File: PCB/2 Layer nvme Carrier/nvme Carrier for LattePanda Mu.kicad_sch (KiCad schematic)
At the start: 8 parts

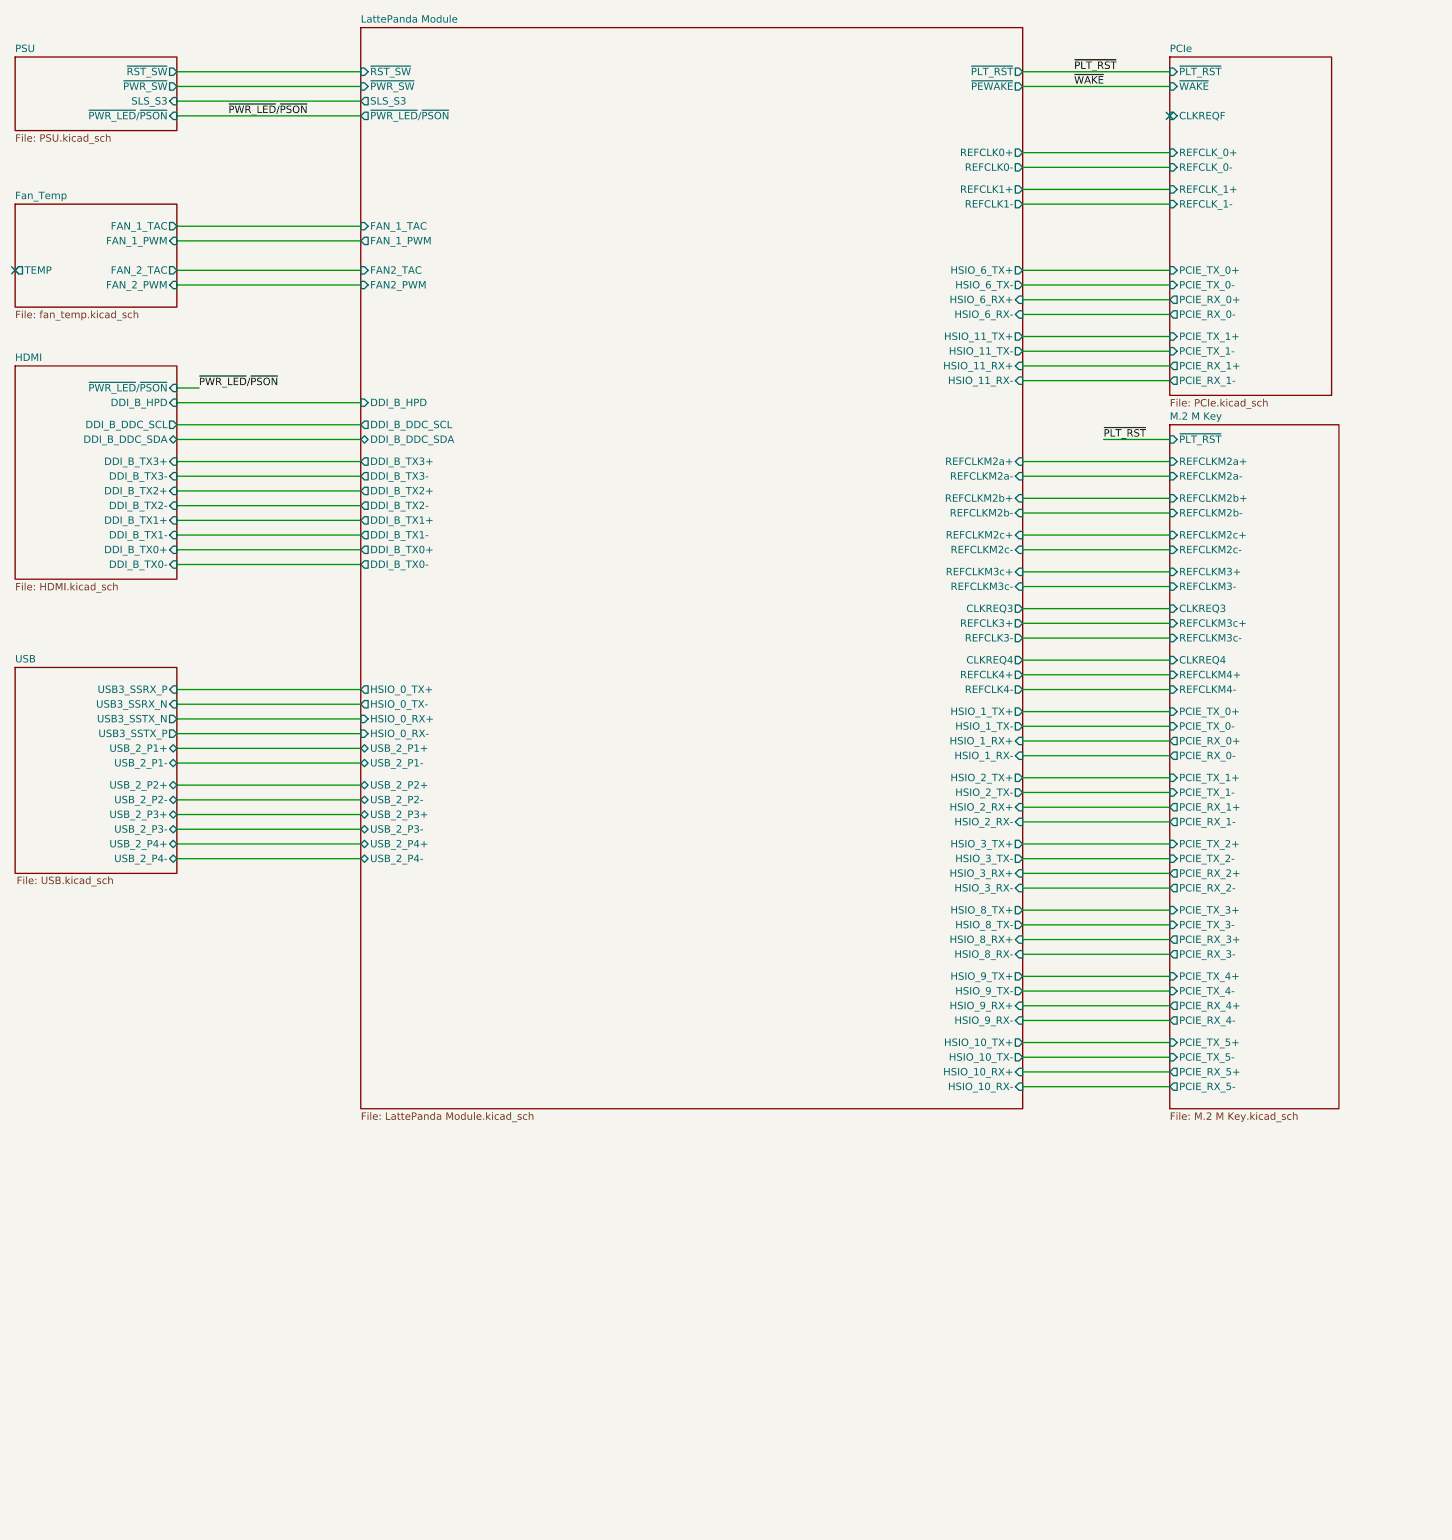
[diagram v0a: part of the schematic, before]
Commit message: Rework started with PCIe
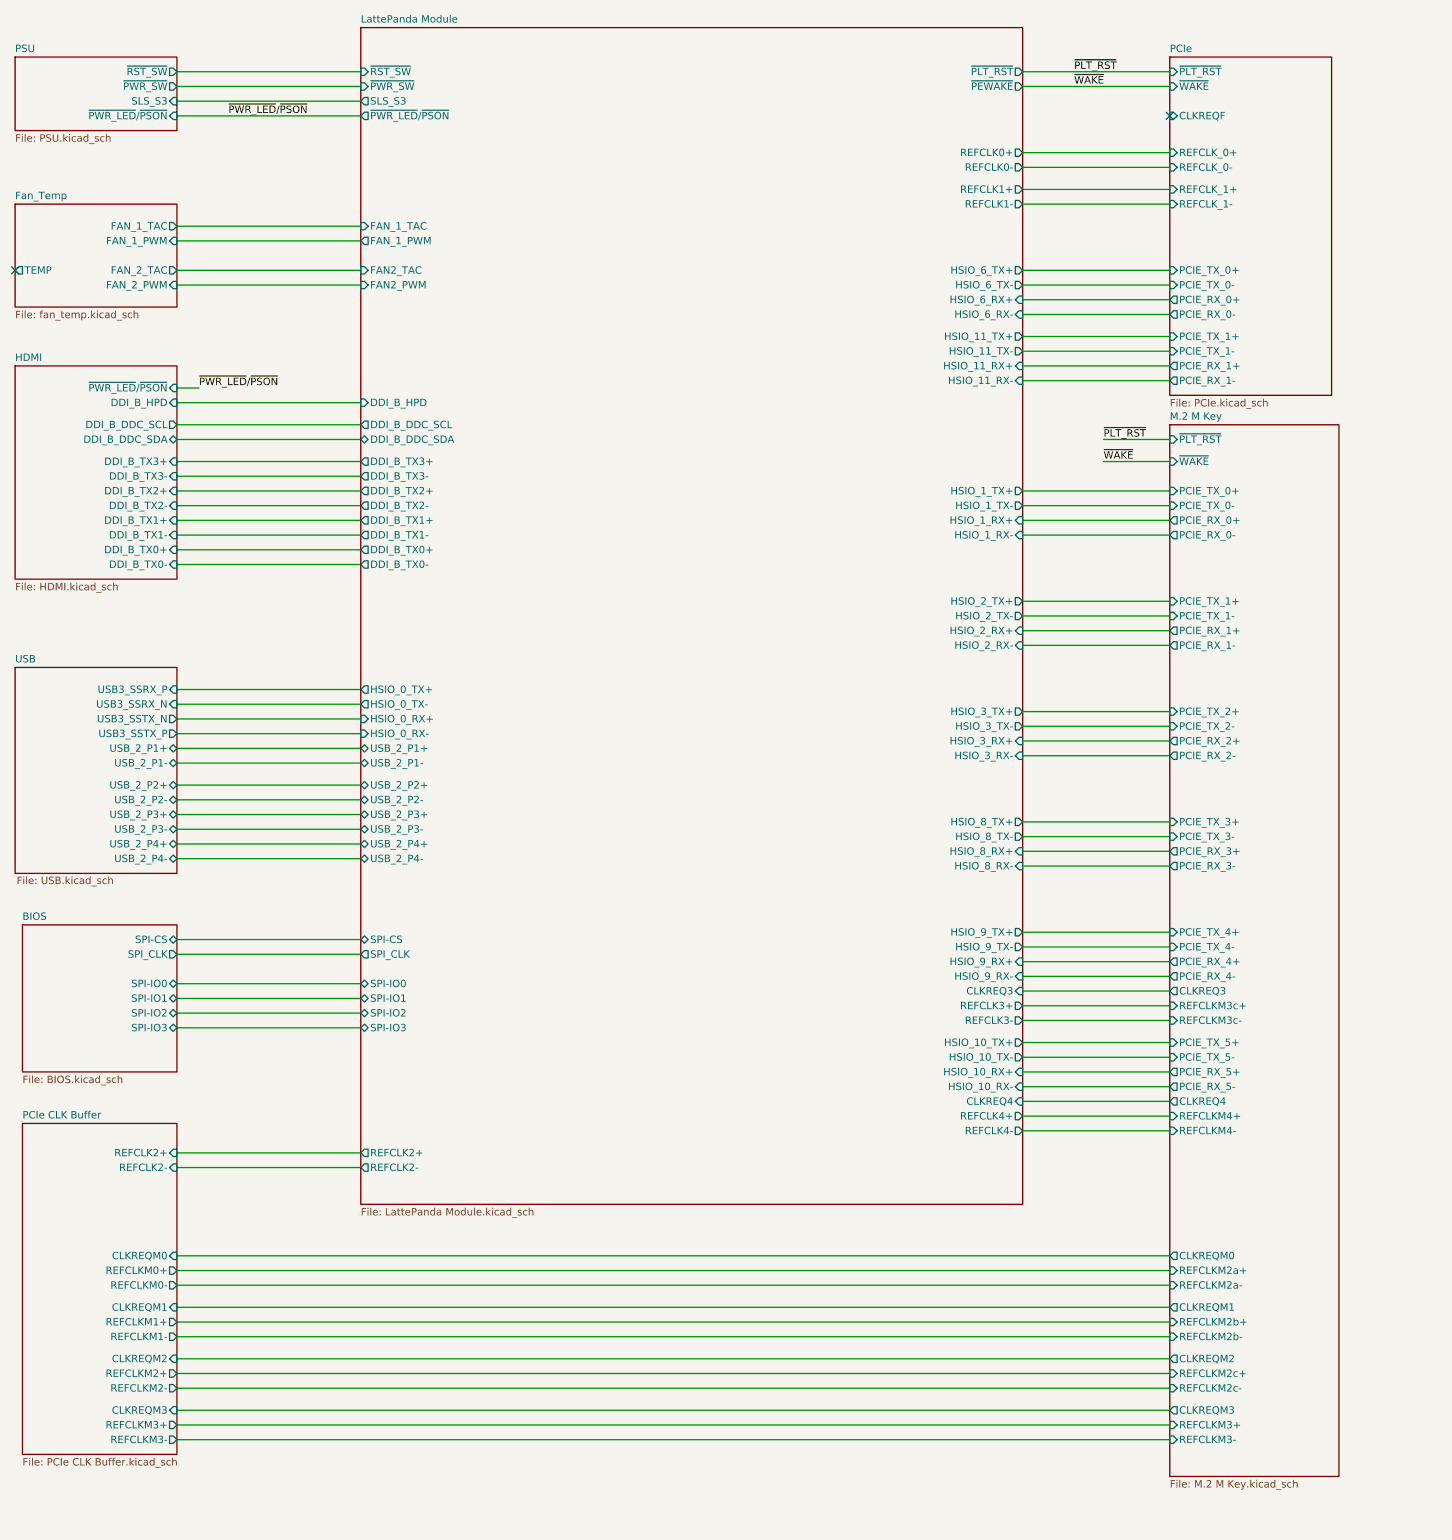
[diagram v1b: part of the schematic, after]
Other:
- added sheet BIOS (BIOS.kicad_sch)
- added sheet PCIe CLK Buffer (PCIe CLK Buffer.kicad_sch)
- sheet LattePanda Module ports: added REFCLK2+, REFCLK2-, SPI-CS, SPI-IO0, SPI-IO1, SPI-IO2, SPI-IO3, SPI_CLK; removed REFCLKM2a+, REFCLKM2a-, REFCLKM2b+, REFCLKM2b-, REFCLKM2c+, REFCLKM2c-, REFCLKM3c+, REFCLKM3c-
- sheet M.2 M Key ports: added CLKREQM0, CLKREQM1, CLKREQM2, CLKREQM3, ~{WAKE}; removed none
